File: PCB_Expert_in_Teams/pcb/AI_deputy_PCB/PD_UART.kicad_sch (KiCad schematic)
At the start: 1 part, among them J2 Battery Input

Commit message: updating repo from desktop
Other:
- company: (none) -> Area 42 & Albers-Online Psykologi
- title: (none) -> AI Deputy
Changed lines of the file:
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@@
 	(generator_version "9.0")
 	(paper "A4")
+	(title_block
+		(title "AI Deputy")
+		(date "2025-09-24")
+		(rev "v0.1")
+		(company "Area 42 & Albers-Online Psykologi")
+		(comment 1 "SDU")
+		(comment 2 "Expert In Teams Semester Project")
+	)
 	(text_box "Battery input from BMS\n"
 		(exclude_from_sim no)

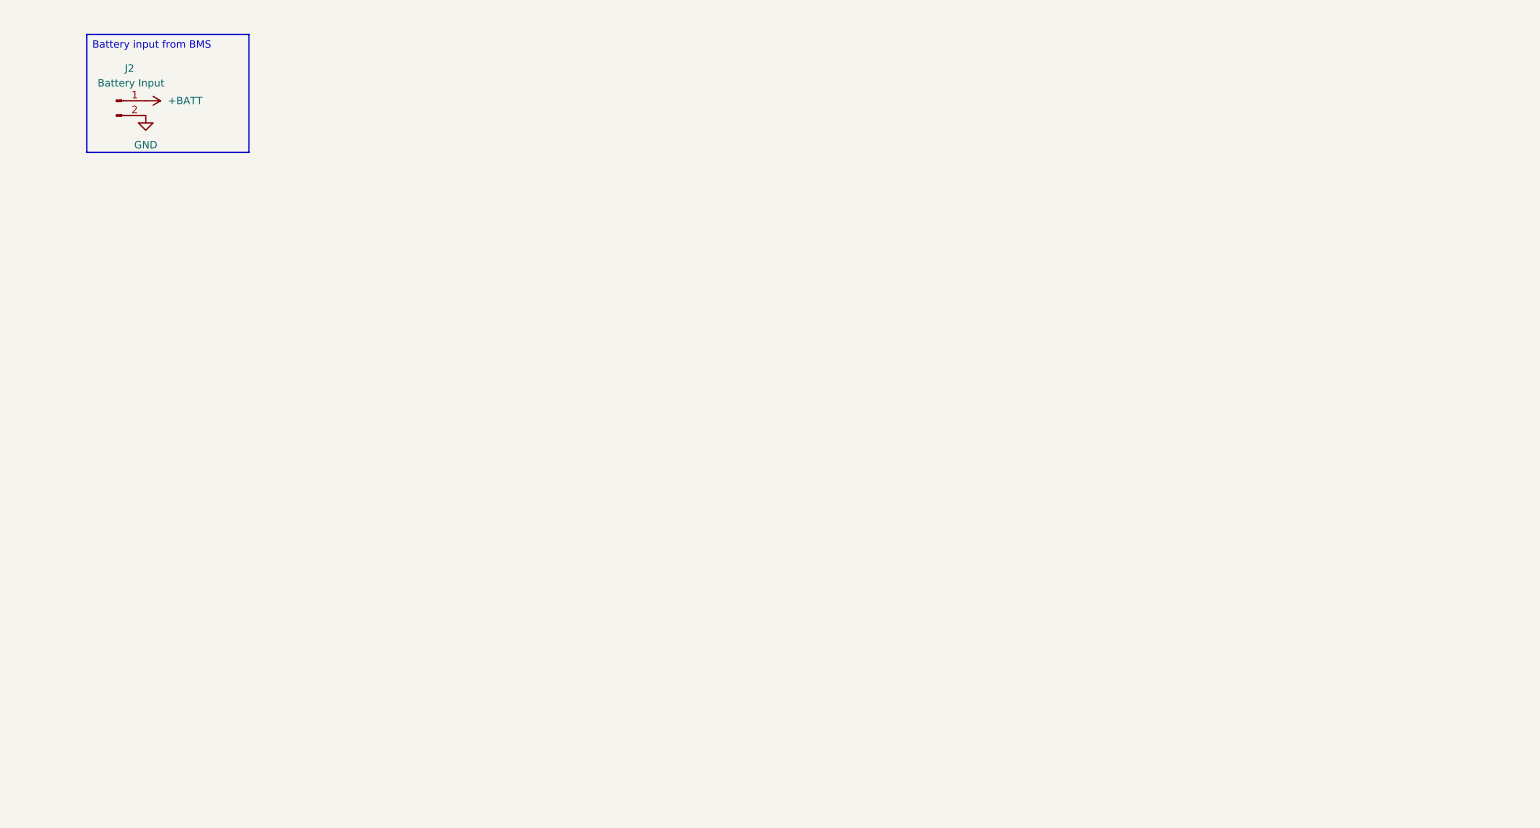
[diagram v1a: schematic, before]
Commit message: 29/10/update
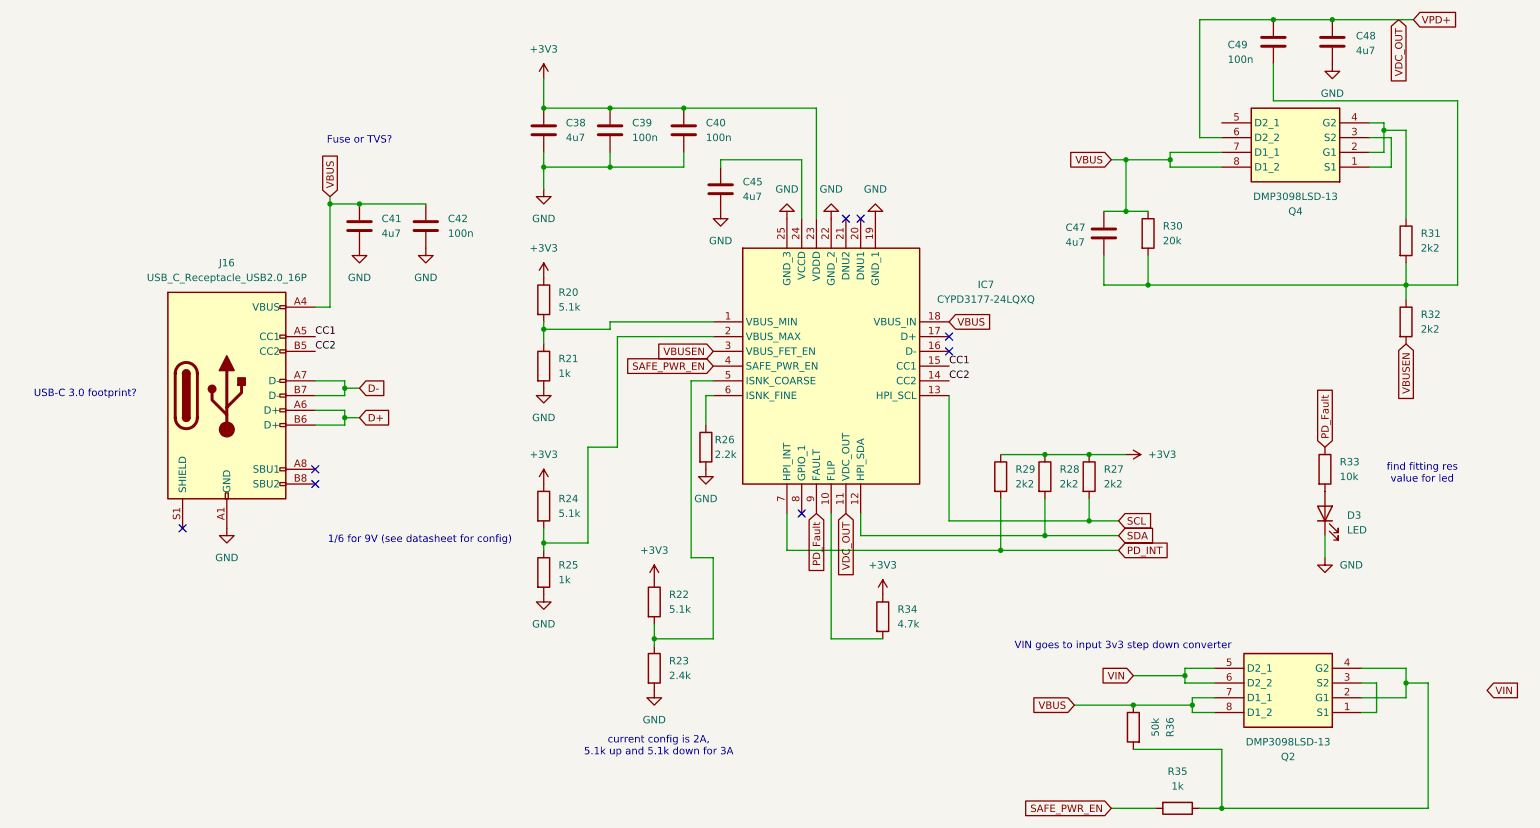
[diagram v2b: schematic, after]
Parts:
- removed J2: Battery Input, symbol Connector:Conn_01x02_Pin
- added C38, C41, C45, C47, C48: 4u7, symbol Device:C
- added C39, C40, C42, C49: 100n, symbol Device:C
- added D3: LED, LED_SMD:LED_0805_2012Metric_Pad1.15x1.40mm_HandSolder, symbol Device:LED
- added IC7: CYPD3177-24LQXQ, QFN50P400X400X60-25N-D, symbol CYPD3177-24LQXQ:CYPD3177-24LQXQ
- added J16: USB_C_Receptacle_USB2.0_16P, EXT_AI_DEPUTY_Library:MOLEX_1054500101, symbol Connector:USB_C_Receptacle_USB2.0_16P
- added Q2, Q4: DMP3098LSD-13, SOIC127P600X175-8N, symbol DMP3098LSD:DMP3098LSD-13
- added R20, R22, R24: 5.1k, Resistor_SMD:R_0805_2012Metric_Pad1.20x1.40mm_HandSolder, symbol Device:R
- added R21, R25, R35: 1k, Resistor_SMD:R_0805_2012Metric_Pad1.20x1.40mm_HandSolder, symbol Device:R
- added R23: 2.4k, Resistor_SMD:R_0805_2012Metric_Pad1.20x1.40mm_HandSolder, symbol Device:R
- added R26: 2.2k, Resistor_SMD:R_0805_2012Metric_Pad1.20x1.40mm_HandSolder, symbol Device:R
- added R27, R28, R29, R31, R32: 2k2, symbol Device:R
- added R30: 20k, symbol Device:R
- added R33: 10k, Resistor_SMD:R_0805_2012Metric_Pad1.20x1.40mm_HandSolder, symbol Device:R
- added R34: 4.7k, Resistor_SMD:R_0805_2012Metric_Pad1.20x1.40mm_HandSolder, symbol Device:R
- added R36: 50k, Resistor_SMD:R_0805_2012Metric_Pad1.20x1.40mm_HandSolder, symbol Device:R
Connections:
- net GND: now also C38.2, C39.2, C40.2, C41.2, C42.2, C45.2, C48.2, D3.1 (K), IC7.19 (GND_1), IC7.22 (GND_2), IC7.25 (GND_3), J16.A1 (GND), J16.A12 (GND), J16.B1 (GND), J16.B12 (GND), R21.2, R23.2, R25.2, R26.2
- new net: C45.1, IC7.24 (VCCD)
- new net: C47.2, C49.2, R30.2, R31.2, R32.1
- new net: IC7.10 (FLIP), R34.2
- new net: IC7.1 (VBUS_MIN), R20.2, R21.1
- new net: IC7.5 (ISNK_COARSE), R22.2, R23.1
- new net: D3.2 (A), R33.2
- new net: Q4.1 (S1), Q4.3 (S2)
- new net: Q4.2 (G1), Q4.4 (G2), R31.1
- new net: IC7.2 (VBUS_MAX), R24.2, R25.1
- new net: IC7.6 (ISNK_FINE), R26.1
- new net: Q2.1 (S1), Q2.3 (S2)
- new net: Q2.2 (G1), Q2.4 (G2), R35.1, R36.2
- new net +3V3: C38.1, C39.1, C40.1, IC7.23 (VDDD), R20.1, R22.1, R24.1, R27.1, R28.1, R29.1, R34.1
- new net CC1: IC7.15 (CC1), J16.A5 (CC1)
- new net CC2: IC7.14 (CC2), J16.B5 (CC2)
- new net D+: J16.A6 (D+), J16.B6 (D+)
- new net D-: J16.A7 (D-), J16.B7 (D-)
- new net PD_Fault: IC7.9 (FAULT), R33.1
- new net PD_INT: IC7.7 (HPI_INT), R29.2
- new net SAFE_PWR_EN: IC7.4 (SAFE_PWR_EN), R35.2
- new net SCL: IC7.13 (HPI_SCL), R27.2
- new net SDA: IC7.12 (HPI_SDA), R28.2
- new net VBUS: C41.1, C42.1, C47.1, IC7.18 (VBUS_IN), J16.A4 (VBUS), J16.A9 (VBUS), J16.B4 (VBUS), J16.B9 (VBUS), Q2.7 (D1_1), Q2.8 (D1_2), Q4.7 (D1_1), Q4.8 (D1_2), R30.1, R36.1
- new net VBUSEN: IC7.3 (VBUS_FET_EN), R32.2
- new net VDC_OUT: C48.1, C49.1, IC7.11 (VDC_OUT), Q4.6 (D2_2)
- new net VIN: Q2.5 (D2_1), Q2.6 (D2_2)
- no-connect marks 0 -> 8
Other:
- note added: "1/6 for 9V (see datasheet for config)"
- note added: "Fuse or TVS?"
- note added: "USB-C 3.0 footprint?"
- note added: "VIN goes to input 3v3 step down converter"
- note added: "current config is 2A, 5.1k up and 5.1k down for 3A"
- note added: "find fitting res value for led"
